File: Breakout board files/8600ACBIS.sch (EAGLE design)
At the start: 9 parts, among them IC1 SI8600AC-B-IS

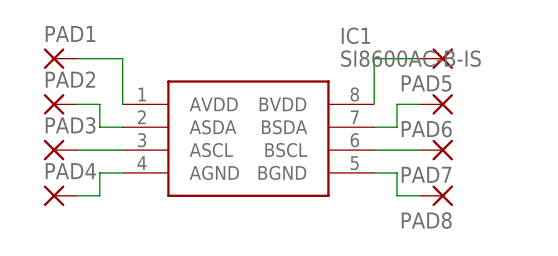
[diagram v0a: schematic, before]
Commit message: Breakout Board Solutions
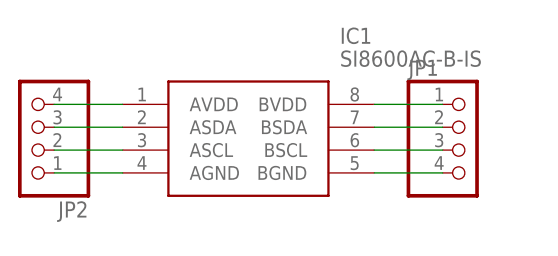
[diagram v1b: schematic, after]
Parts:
- removed PAD1, PAD2, PAD3, PAD4, PAD5, PAD6, PAD7, PAD8: (no value), ee2parts:PAD-TERMINAL
- added JP1, JP2: (no value), pinhead:PINHD-1X4
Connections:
- net N$1: now also JP2.4; no longer PAD1.P
- net N$2: now also JP2.3; no longer PAD2.P
- net N$3: now also JP2.2; no longer PAD3.P
- net N$4: now also JP2.1; no longer PAD4.P
- net N$5: now also IC1.BVDD, JP1.1; no longer IC1.BGND, PAD8.P
- net N$6: now also IC1.BSDA, JP1.2; no longer IC1.BSCL, PAD7.P
- net N$7: now also IC1.BSCL, JP1.3; no longer IC1.BSDA, PAD6.P
- net N$8: now also IC1.BGND, JP1.4; no longer IC1.BVDD, PAD5.P
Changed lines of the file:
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@@
 <?xml version="1.0" encoding="utf-8"?>
 <!DOCTYPE eagle SYSTEM "eagle.dtd">
-<eagle version="8.3.2">
+<eagle version="9.2.0">
 <drawing>
 <settings>
@@
 <layers>
 <layer number="1" name="Top" color="4" fill="1" visible="no" active="no"/>
+<layer number="2" name="Route2" color="1" fill="3" visible="no" active="no"/>
+<layer number="3" name="Route3" color="4" fill="3" visible="no" active="no"/>
+<layer number="4" name="Route4" color="1" fill="4" visible="no" active="no"/>
+<layer number="5" name="Route5" color="4" fill="4" visible="no" active="no"/>
+<layer number="6" name="Route6" color="1" fill="8" visible="no" active="no"/>
+<layer number="7" name="Route7" color="4" fill="8" visible="no" active="no"/>
+<layer number="8" name="Route8" color="1" fill="2" visible="no" active="no"/>
+<layer number="9" name="Route9" color="4" fill="2" visible="no" active="no"/>
+<layer number="10" name="Route10" color="1" fill="7" visible="no" active="no"/>
+<layer number="11" name="Route11" color="4" fill="7" visible="no" active="no"/>
+<layer number="12" name="Route12" color="1" fill="5" visible="no" active="no"/>
+<layer number="13" name="Route13" color="4" fill="5" visible="no" active="no"/>
+<layer number="14" name="Route14" color="1" fill="6" visible="no" active="no"/>
+<layer number="15" name="Route15" color="4" fill="6" visible="no" active="no"/>
 <layer number="16" name="Bottom" color="1" fill="1" visible="no" active="no"/>
 <layer number="17" name="Pads" color="2" fill="1" visible="no" active="no"/>
@@
 <parts>
 <part name="IC1" library="Si8600AC-B-IS" deviceset="SI8600AC-B-IS" device=""/>
-<part name="PAD1" library="ee2parts" deviceset="PAD-TERMINAL" device=""/>
-<part name="PAD2" library="ee2parts" deviceset="PAD-TERMINAL" device=""/>
-<part name="PAD3" library="ee2parts" deviceset="PAD-TERMINAL" device=""/>
-<part name="PAD4" library="ee2parts" deviceset="PAD-TERMINAL" device=""/>
-<part name="PAD5" library="ee2parts" deviceset="PAD-TERMINAL" device=""/>
-<part name="PAD6" library="ee2parts" deviceset="PAD-TERMINAL" device=""/>
-<part name="PAD7" library="ee2parts" deviceset="PAD-TERMINAL" device=""/>
-<part name="PAD8" library="ee2parts" deviceset="PAD-TERMINAL" device=""/>
+<part name="JP1" library="pinhead" library_urn="urn:adsk.eagle:library:325" deviceset="PINHD-1X4" device="" package3d_urn="urn:adsk.eagle:package:22407/2"/>
+<part name="JP2" library="pinhead" library_urn="urn:adsk.eagle:library:325" deviceset="PINHD-1X4" device="" package3d_urn="urn:adsk.eagle:package:22407/2"/>
 </parts>
 <sheets>
@@
 </plain>
 <instances>
-<instance part="IC1" gate="G$1" x="53.34" y="50.8"/>
-<instance part="PAD1" gate="1" x="45.72" y="55.88"/>
-<instance part="PAD2" gate="1" x="45.72" y="50.8"/>
-<instance part="PAD3" gate="1" x="45.72" y="45.72"/>
-<instance part="PAD4" gate="1" x="45.72" y="40.64"/>
-<instance part="PAD5" gate="1" x="88.9" y="55.88" rot="R180"/>
-<instance part="PAD6" gate="1" x="88.9" y="50.8" rot="R180"/>
-<instance part="PAD7" gate="1" x="88.9" y="45.72" rot="R180"/>
-<instance part="PAD8" gate="1" x="88.9" y="40.64" rot="R180"/>
+<instance part="IC1" gate="G$1" x="53.34" y="50.8">
+<attribute name="NAME" x="77.47" y="58.42" size="1.778" layer="95" align="center-left"/>
+<attribute name="VALUE" x="77.47" y="55.88" size="1.778" layer="96" align="center-left"/>
+</instance>
+<instance part="JP1" gate="A" x="91.44" y="45.72">
+<attribute name="NAME" x="85.09" y="53.975" size="1.778" layer="95"/>
+<attribute name="VALUE" x="85.09" y="38.1" size="1.778" layer="96"/>
+</instance>
+<instance part="JP2" gate="A" x="43.18" y="48.26" rot="R180">
+<attribute name="NAME" x="49.53" y="40.005" size="1.778" layer="95" rot="R180"/>
+<attribute name="VALUE" x="49.53" y="55.88" size="1.778" layer="96" rot="R180"/>
+</instance>
 </instances>
 <busses>
@@
 <segment>
 <pinref part="IC1" gate="G$1" pin="AVDD"/>
-<wire x1="53.34" y1="50.8" x2="53.34" y2="55.88" width="0.1524" layer="91"/>
-<pinref part="PAD1" gate="1" pin="P"/>
-<wire x1="53.34" y1="55.88" x2="48.26" y2="55.88" width="0.1524" layer="91"/>
+<pinref part="JP2" gate="A" pin="4"/>
+<wire x1="53.34" y1="50.8" x2="45.72" y2="50.8" width="0.1524" layer="91"/>
 </segment>
 </net>
 <net name="N$2" class="0">
 <segment>
+<pinref part="JP2" gate="A" pin="3"/>
 <pinref part="IC1" gate="G$1" pin="ASDA"/>
-<wire x1="53.34" y1="48.26" x2="50.8" y2="48.26" width="0.1524" layer="91"/>
-<wire x1="50.8" y1="48.26" x2="50.8" y2="50.8" width="0.1524" layer="91"/>
-<pinref part="PAD2" gate="1" pin="P"/>
-<wire x1="50.8" y1="50.8" x2="48.26" y2="50.8" width="0.1524" layer="91"/>
+<wire x1="45.72" y1="48.26" x2="53.34" y2="48.26" width="0.1524" layer="91"/>
 </segment>
 </net>
 <net name="N$3" class="0">
 <segment>
+<pinref part="JP2" gate="A" pin="2"/>
 <pinref part="IC1" gate="G$1" pin="ASCL"/>
-<pinref part="PAD3" gate="1" pin="P"/>
-<wire x1="53.34" y1="45.72" x2="48.26" y2="45.72" width="0.1524" layer="91"/>
+<wire x1="45.72" y1="45.72" x2="53.34" y2="45.72" width="0.1524" layer="91"/>
 </segment>
 </net>
 <net name="N$4" class="0">
 <segment>
+<pinref part="JP2" gate="A" pin="1"/>
 <pinref part="IC1" gate="G$1" pin="AGND"/>
-<wire x1="53.34" y1="43.18" x2="50.8" y2="43.18" width="0.1524" layer="91"/>
-<wire x1="50.8" y1="43.18" x2="50.8" y2="40.64" width="0.1524" layer="91"/>
-<pinref part="PAD4" gate="1" pin="P"/>
-<wire x1="50.8" y1="40.64" x2="48.26" y2="40.64" width="0.1524" layer="91"/>
+<wire x1="45.72" y1="43.18" x2="53.34" y2="43.18" width="0.1524" layer="91"/>
 </segment>
 </net>
 <net name="N$5" class="0">
 <segment>
-<pinref part="IC1" gate="G$1" pin="BGND"/>
-<wire x1="81.28" y1="43.18" x2="83.82" y2="43.18" width="0.1524" layer="91"/>
-<wire x1="83.82" y1="43.18" x2="83.82" y2="40.64" width="0.1524" layer="91"/>
-<pinref part="PAD8" gate="1" pin="P"/>
-<wire x1="83.82" y1="40.64" x2="86.36" y2="40.64" width="0.1524" layer="91"/>
+<pinref part="IC1" gate="G$1" pin="BVDD"/>
+<pinref part="JP1" gate="A" pin="1"/>
+<wire x1="81.28" y1="50.8" x2="88.9" y2="50.8" width="0.1524" layer="91"/>
 </segment>
 </net>
 <net name="N$6" class="0">
 <segment>
-<pinref part="PAD7" gate="1" pin="P"/>
-<pinref part="IC1" gate="G$1" pin="BSCL"/>
-<wire x1="86.36" y1="45.72" x2="81.28" y2="45.72" width="0.1524" layer="91"/>
+<pinref part="JP1" gate="A" pin="2"/>
+<pinref part="IC1" gate="G$1" pin="BSDA"/>
+<wire x1="88.9" y1="48.26" x2="81.28" y2="48.26" width="0.1524" layer="91"/>
 </segment>
 </net>
 <net name="N$7" class="0">
 <segment>
-<pinref part="PAD6" gate="1" pin="P"/>
-<wire x1="86.36" y1="50.8" x2="83.82" y2="50.8" width="0.1524" layer="91"/>
-<wire x1="83.82" y1="50.8" x2="83.82" y2="48.26" width="0.1524" layer="91"/>
-<pinref part="IC1" gate="G$1" pin="BSDA"/>
-<wire x1="83.82" y1="48.26" x2="81.28" y2="48.26" width="0.1524" layer="91"/>
+<pinref part="IC1" gate="G$1" pin="BSCL"/>
+<pinref part="JP1" gate="A" pin="3"/>
+<wire x1="81.28" y1="45.72" x2="88.9" y2="45.72" width="0.1524" layer="91"/>
 </segment>
 </net>
 <net name="N$8" class="0">
 <segment>
-<pinref part="PAD5" gate="1" pin="P"/>
-<pinref part="IC1" gate="G$1" pin="BVDD"/>
-<wire x1="86.36" y1="55.88" x2="81.28" y2="55.88" width="0.1524" layer="91"/>
-<wire x1="81.28" y1="55.88" x2="81.28" y2="50.8" width="0.1524" layer="91"/>
+<pinref part="JP1" gate="A" pin="4"/>
+<pinref part="IC1" gate="G$1" pin="BGND"/>
+<wire x1="88.9" y1="43.18" x2="81.28" y2="43.18" width="0.1524" layer="91"/>
 </segment>
 </net>
@@
 </schematic>
 </drawing>
+<compatibility>
+<note version="8.2" severity="warning">
+Since Version 8.2, EAGLE supports online libraries. The ids
+of those online libraries will not be understood (or retained)
+with this version.
+</note>
+<note version="8.3" severity="warning">
+Since Version 8.3, EAGLE supports URNs for individual library
+assets (packages, symbols, and devices). The URNs of those assets
+will not be understood (or retained) with this version.
+</note>
+<note version="8.3" severity="warning">
+Since Version 8.3, EAGLE supports the association of 3D packages
+with devices in libraries, schematics, and board files. Those 3D
+packages will not be understood (or retained) with this version.
+</note>
+</compatibility>
 </eagle>
